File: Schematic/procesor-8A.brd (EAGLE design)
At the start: 27.9 x 27.9 mm, 5 parts

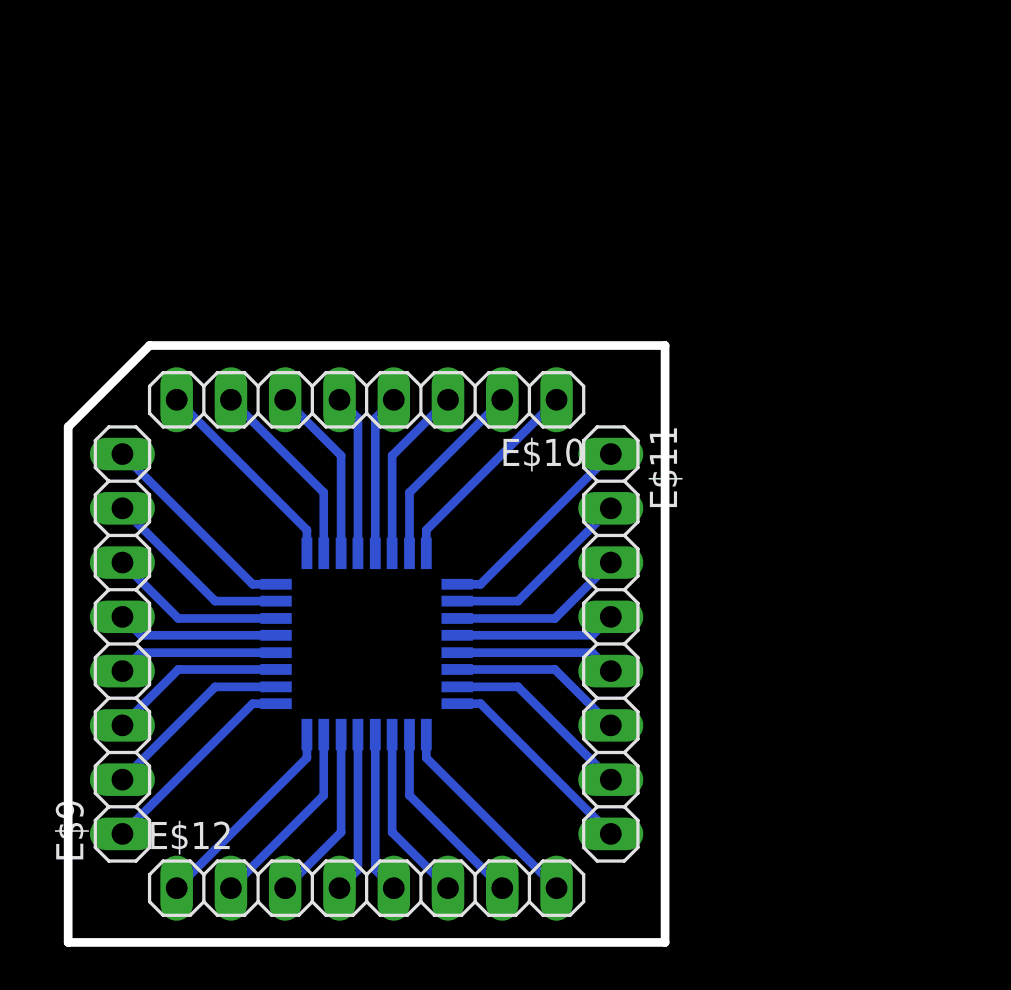
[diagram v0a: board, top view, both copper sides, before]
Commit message: Add files via upload
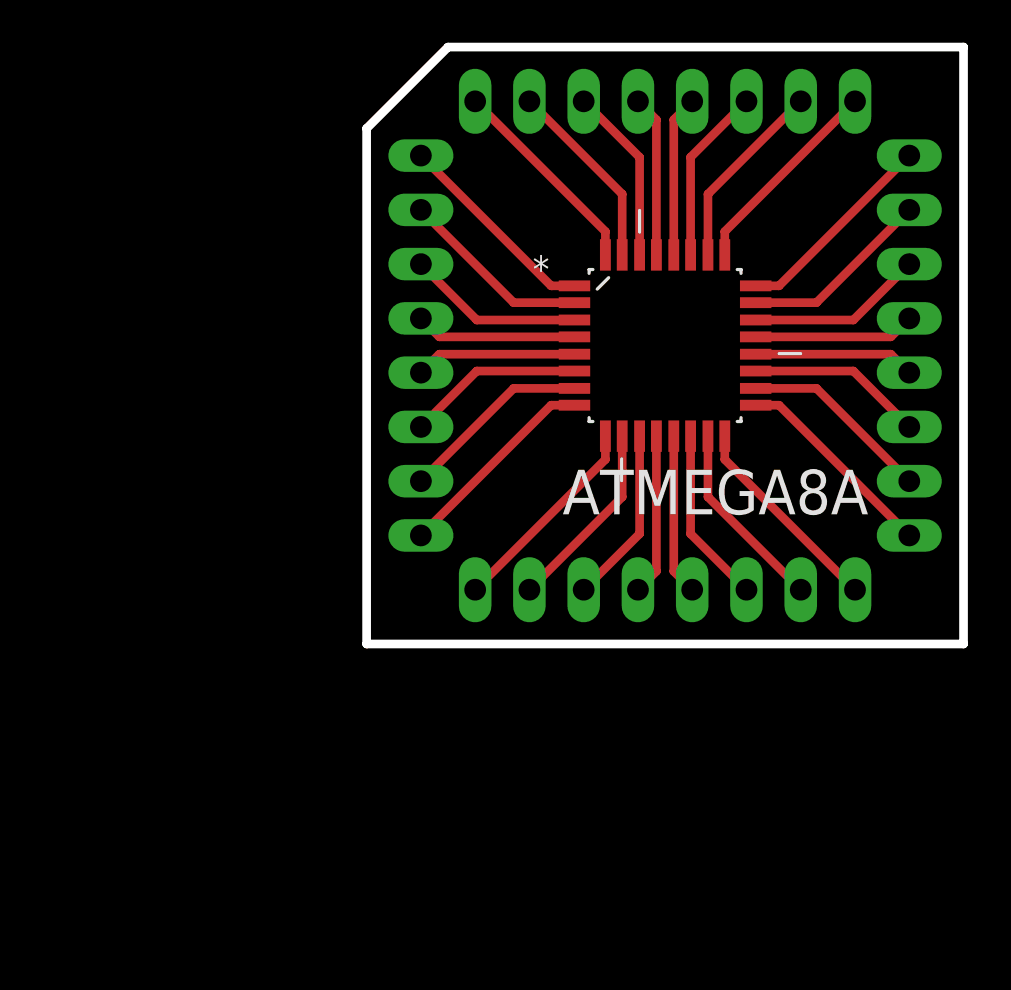
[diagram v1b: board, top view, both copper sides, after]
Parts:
- moved E$12 35.9 mm to (25.4, 14.0), flipped to the bottom, turned to 270 degrees
- moved E$9 35.9 mm to (14.0, 25.4), flipped to the bottom, turned to 0 degrees
- moved ATMEGA8A 19.8 mm to (14.0, 14.0), flipped to the top, turned to 0 degrees
- moved E$10 3.59 mm to (2.54, 14.0), flipped to the bottom, turned to 90 degrees
- moved E$11 3.59 mm to (14.0, 2.54), flipped to the bottom, turned to 180 degrees
